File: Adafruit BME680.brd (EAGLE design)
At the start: 17.8 x 16.5 mm, 17 parts, among them Q1 2N7002D, U1 BME280, U2 MIC5225-3.3

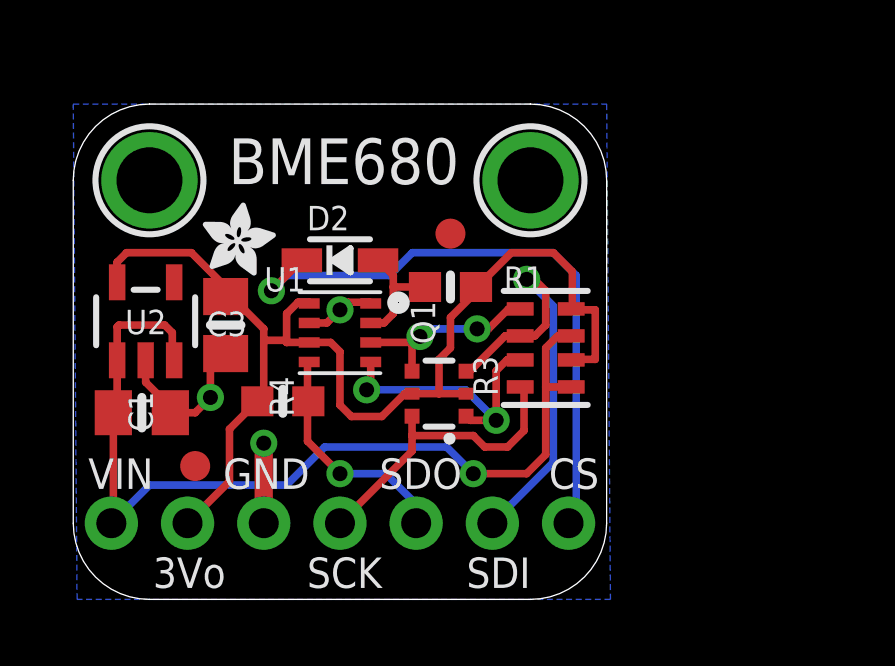
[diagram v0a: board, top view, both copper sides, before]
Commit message: Updated PCB files
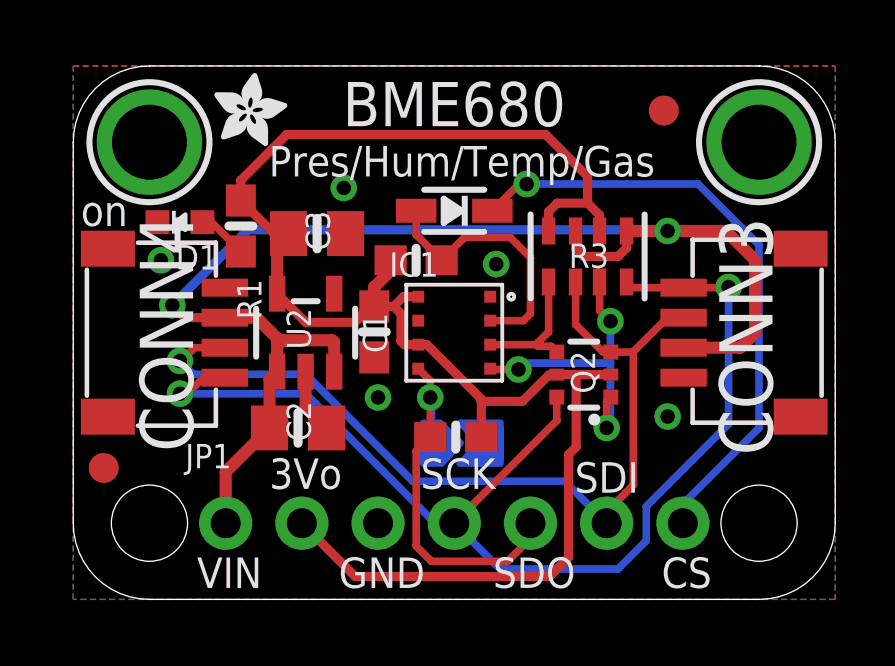
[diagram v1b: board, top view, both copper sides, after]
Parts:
- removed JP2: (no value), microbuilder:1X07_ROUND_70
- removed Q1: 2N7002D, microbuilder:SOT363
- removed U$15, U$5: FIDUCIAL_1MM, microbuilder:FIDUCIAL_1MM
- removed U$2, U$6: (no value), microbuilder:ADAFRUIT_2.5MM
- removed U$20: (no value), microbuilder:PCBFEAT-REV-040
- removed U$7, U$8: MOUNTINGHOLE2.0, microbuilder:MOUNTINGHOLE_2.0_PLATED
- removed U1: BME280, microbuilder:BME280
- added C2: 10uF, microbuilder:0805-NO
- added CONN3, CONN4: STEMMA_I2C_QT, microbuilder:JST_SH4
- added D1: GREEN, microbuilder:CHIPLED_0603_NOOUTLINE
- added FID3, FID4: FIDUCIAL_1MM, microbuilder:FIDUCIAL_1MM
- added IC1: BME680, adafruit_sensor:BME680
- added JP1: (no value), microbuilder:1X07_ROUND_70
- added Q2: BSS138, microbuilder:SOT363
- added R5: 10K, microbuilder:0603-NO
- added SJ1: (no value), microbuilder:SOLDERJUMPER_ARROW_NOPASTE
- added U$1, U$17: MOUNTINGHOLE2.5, microbuilder:MOUNTINGHOLE_2.5_PLATED
- added U$25: (no value), microbuilder:PCBFEAT-REV-040
- added U$30, U$31: (no value), silks:STEMMAQT
- added U$4: (no value), microbuilder:ADAFRUIT_2.5MM
- C1: value 10uF -> 0.1uF; device microbuilder:0805-NO -> microbuilder:0603-NO
- U2: value MIC5225-3.3 -> AP2112K-3.3
- moved C1 8.20 mm to (10.0, 8.92), turned to 270 degrees
- moved R1 7.27 mm to (5.59, 12.4), turned to 270 degrees
- moved R4 5.89 mm to (12.8, 5.41), turned to 0 degrees
- moved U2 5.35 mm to (7.75, 8.89)
- moved C3 4.31 mm to (8.13, 12.2), turned to 0 degrees
- moved D2 4.15 mm to (12.7, 13.0), turned to 180 degrees
- moved R3 3.35 mm to (17.1, 11.4), turned to 180 degrees
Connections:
- removed net VIN: C1.1, JP2.1, R3.1, R3.3, U2.1, U2.3
- new net N$1: D1.A, R1.2
- new net VCC: C2.1, CONN3.2, CONN4.2, JP1.1, R3.1, R3.3, U2.1, U2.3
- net 3.3V: now also C1.1, IC1.6, IC1.8, JP1.2, Q2.2, Q2.5, R1.1, R5.2; no longer JP2.2, Q1.2, Q1.5, R1.2, U1.6, U1.8
- net CS: now also JP1.7; no longer JP2.7
- net CS_3V: now also IC1.2, R5.1; no longer R1.1, U1.2
- net GND: now also C2.2, CONN3.1, CONN4.1, D1.C, IC1.1, IC1.7, JP1.3, SJ1.2; no longer JP2.3, U1.1, U1.7
- net SCK/SCL: now also CONN3.4, CONN4.4, JP1.4, Q2.6; no longer JP2.4, Q1.6
- net SCK_3V: now also IC1.4, Q2.1; no longer Q1.1, U1.4
- net SDI/SDA: now also CONN3.3, CONN4.3, JP1.6, Q2.3; no longer JP2.6, Q1.3
- net SDI_3V: now also IC1.3, Q2.4; no longer Q1.4, U1.3
- net SDO/ADR: now also IC1.5, JP1.5, SJ1.1; no longer JP2.5, U1.5
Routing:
- net VCC: track 0.00 -> 44.2 mm, vias 0 -> 2
- net VIN: track 31.3 -> 0.00 mm, vias 1 -> 0
- net SCK/SCL: track 10.2 -> 38.8 mm, vias 0 -> 2
- net 3.3V: track 38.3 -> 55.7 mm
- net SDI/SDA: track 15.0 -> 30.1 mm
- net GND: track 10.3 -> 2.16 mm, vias 3 -> 5
- net CS_3V: track 3.92 -> 8.86 mm
- net SDO/ADR: track 8.09 -> 12.7 mm
- net SDI_3V: track 6.71 -> 4.66 mm, vias 2 -> 0
- net N$1: track 0.00 -> 1.69 mm
- net SCK_3V: track 9.39 -> 10.3 mm, vias 2 -> 3
- net CS: track 21.0 -> 20.4 mm
- added copper zone on layer 1, net GND
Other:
- board size 17.8 x 16.5 mm -> 25.4 x 17.8 mm
- board text added: "Addr"
- board text added: "Default I2C Addr 0x77"
- board text added: "Pres/Hum/Temp/Gas"
- board text added: "Temp, Pressure Humidity & Gas"
- board text added: "VLogic/Vcc: 3-5VDC"
- board text added: "on"
- board text removed: "Barometric Pressure Humidity, Temp & Gas Sensor"
- board text removed: "SPI or I2C"
- board text removed: "Vin/Vlogic: 3-5V"
- board text removed: "adafruit!"
